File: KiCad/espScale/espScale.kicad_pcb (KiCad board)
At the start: 2 copper layers, 73.7 x 64.1 mm, 7 parts, among them J1 2-pin_power_input_header, U1 NodeMCU1.0(ESP-12E), U2 3-wire_Load_Cell, U4 3-wire_Load_Cell, U6 HX711_Load_Cell_Amplifier

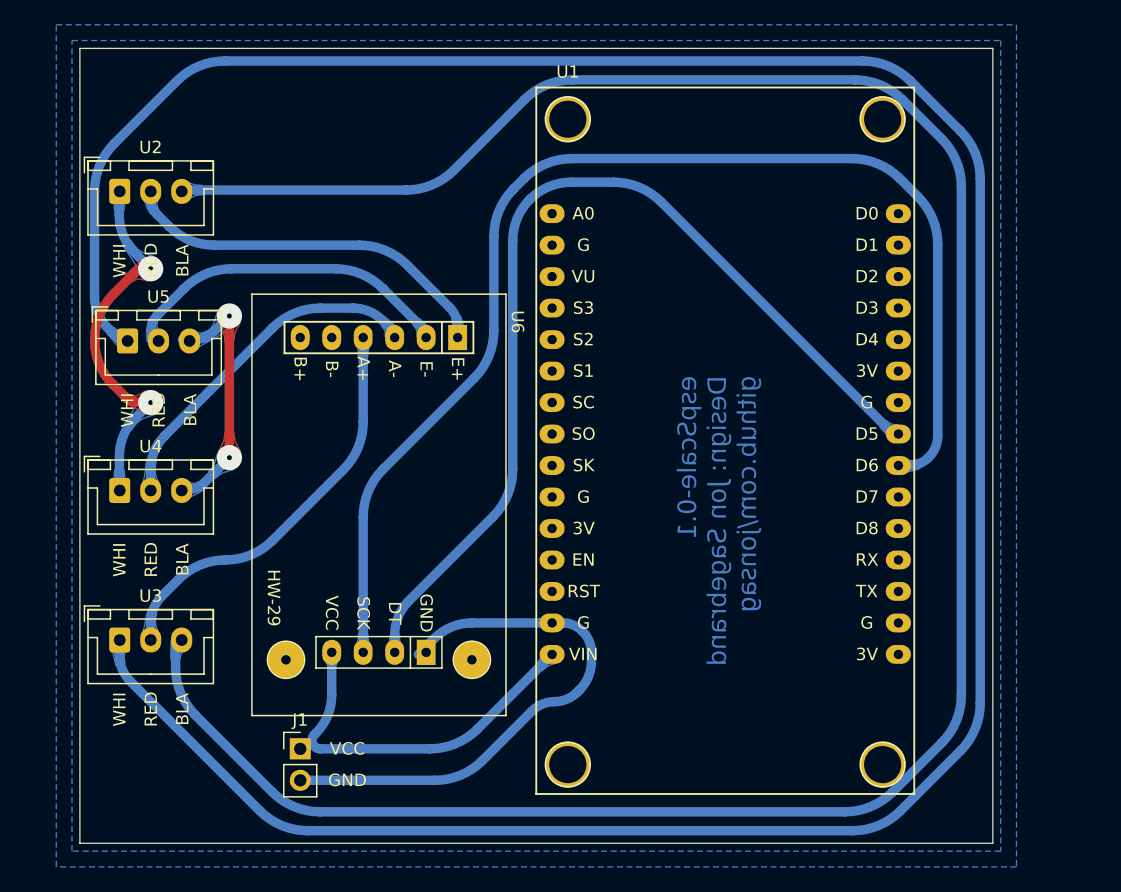
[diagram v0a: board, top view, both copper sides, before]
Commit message: new PCB, added 3-pin LCD
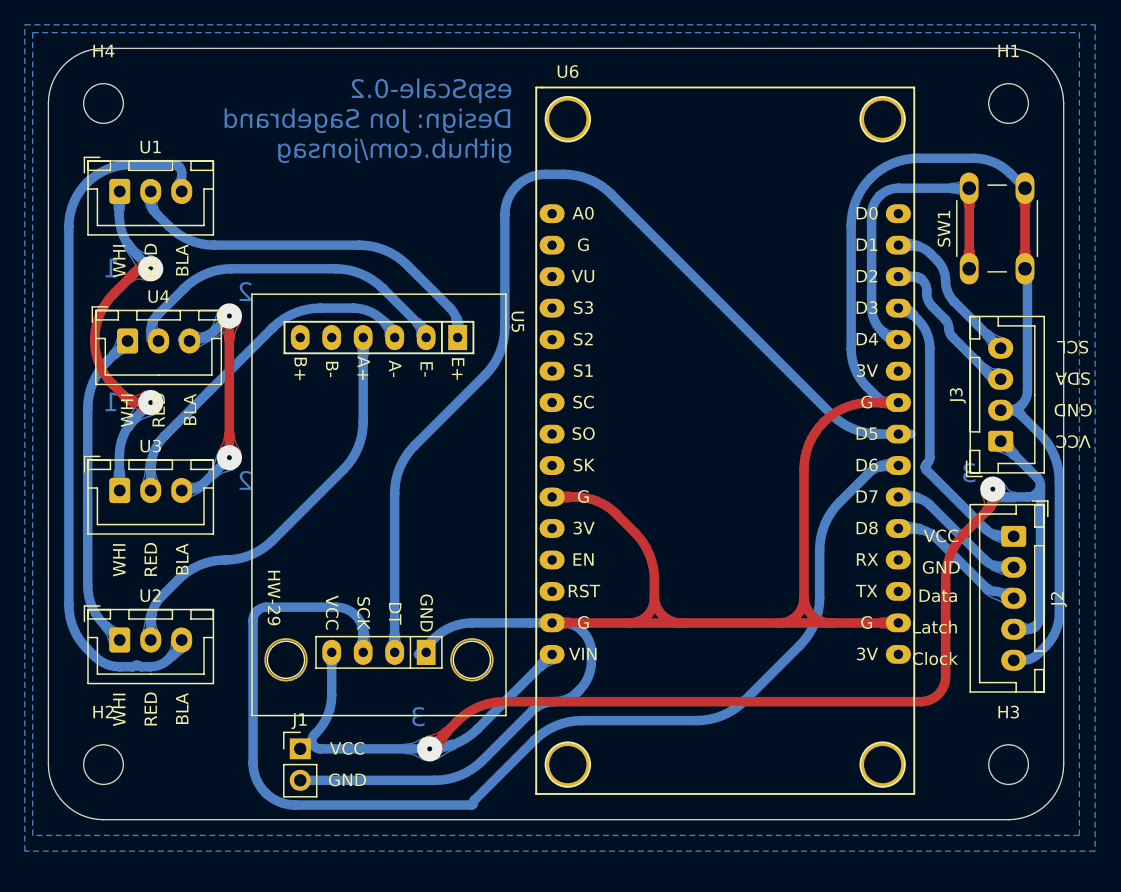
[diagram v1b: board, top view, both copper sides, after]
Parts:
- added H1: MountingHole, MountingHole:MountingHole_3.2mm_M3, F.Cu at (163.8, 66.0)
- added H2: MountingHole, MountingHole:MountingHole_3.2mm_M3, F.Cu at (90.8, 119.4)
- added H3: MountingHole, MountingHole:MountingHole_3.2mm_M3, F.Cu at (163.8, 119.4)
- added H4: MountingHole, MountingHole:MountingHole_3.2mm_M3, F.Cu at (90.8, 66.0)
- added J2: 5-pin_LCD, My_Headers:5-pin JST LiquidCrystal595, F.Cu at (164.2, 101.0)
- added J3: I2C Display, My_Headers:4-pin JST LCD, F.Cu at (163.2, 93.3)
- added SW1: Reset, My_Misc:SW_PUSH_6mm_large, F.Cu at (160.7, 79.4)
- renumbered U2 to U1, U3 to U2, U4 to U3, U5 to U4, U6 to U5, U1 to U6
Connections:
- U6 pad 10: unconnected-(U1-Pad10) -> GND
- U6 pad 17: unconnected-(U1-Pad17) -> GND
- U6 pad 20: unconnected-(U1-Pad20) -> Clock
- U6 pad 21: unconnected-(U1-Pad21) -> Latch
- U6 pad 24: unconnected-(U1-Pad24) -> GND
- U6 pad 26: unconnected-(U1-Pad26) -> Net-(U6-Pad26)
- U6 pad 27: unconnected-(U1-Pad27) -> Data
- U6 pad 28: unconnected-(U1-Pad28) -> SDA
- U6 pad 29: unconnected-(U1-Pad29) -> SCL
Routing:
- net Net-(U2-Pad1): track 218.3 -> 26.1 mm
- net GND: track 44.5 -> 198.2 mm
- net Net-(U1-Pad3): track 187.5 -> 57.4 mm
- net +5V: track 30.6 -> 114.0 mm, vias 0 -> 2
- net Net-(U6-Pad26): track 0.00 -> 26.7 mm
- net Data: track 0.00 -> 23.6 mm
- net SDA: track 0.00 -> 12.6 mm
- net SCL: track 0.00 -> 12.5 mm
- net Latch: track 0.00 -> 11.4 mm
- net Clock: track 0.00 -> 11.4 mm
- net SCK: track 100.2 -> 92.8 mm
- net DT: track 78.8 -> 81.2 mm
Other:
- board size 73.7 x 64.1 mm -> 81.9 x 62.2 mm
- board text added: "1"
- board text added: "2"
- board text added: "3"
